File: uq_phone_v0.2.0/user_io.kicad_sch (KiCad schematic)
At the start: 23 parts, among them J8 MCS-302S-C1, M1 C08-00A, Q3 S8050, Q6 MMBT3904LP-7, U10 TPD8F003DQDR, U11 LSM6DSVTR, U12 DRV2603RUNR, U7 TPS22964CYZPR, U8 TPD3F303DQDR

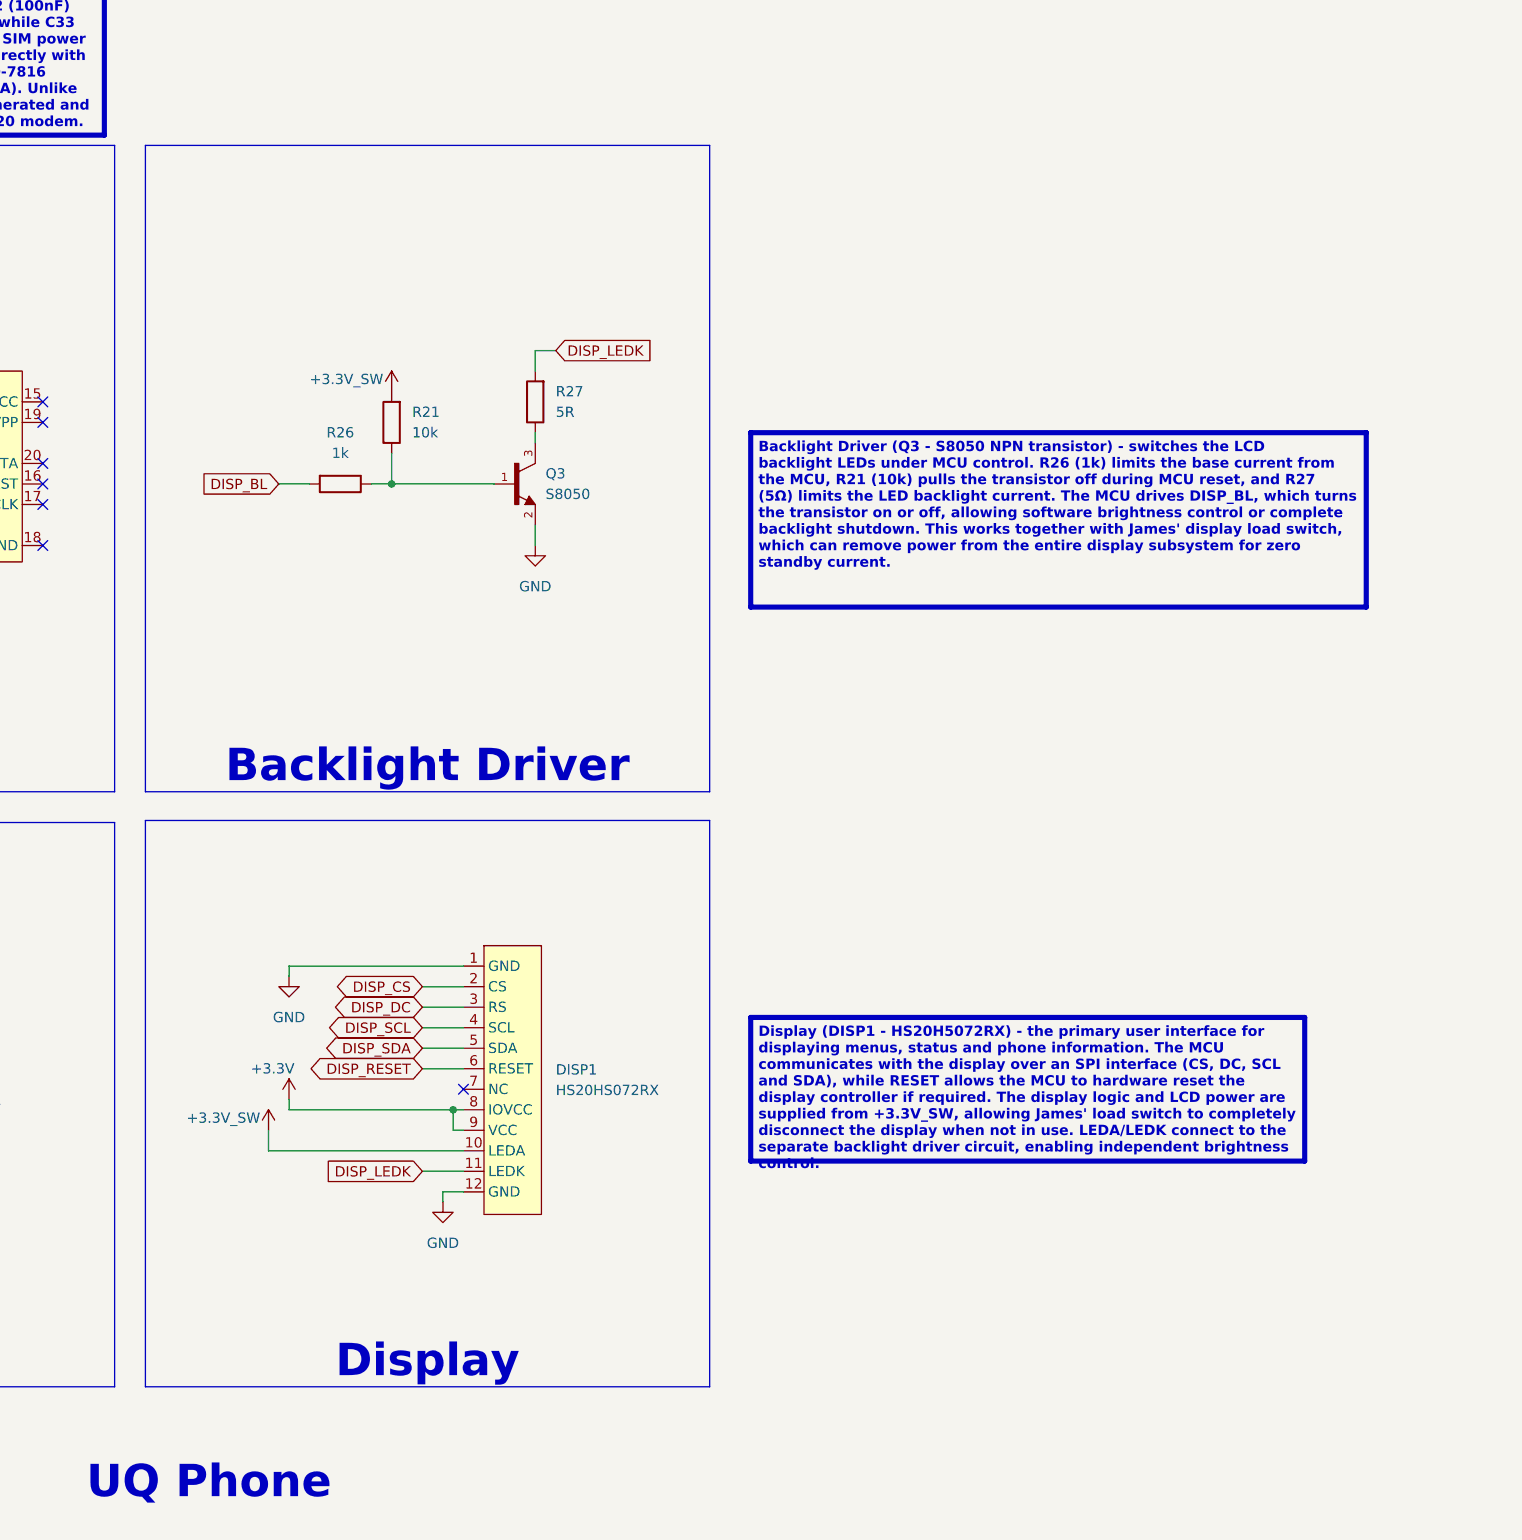
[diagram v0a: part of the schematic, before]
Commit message: new display work
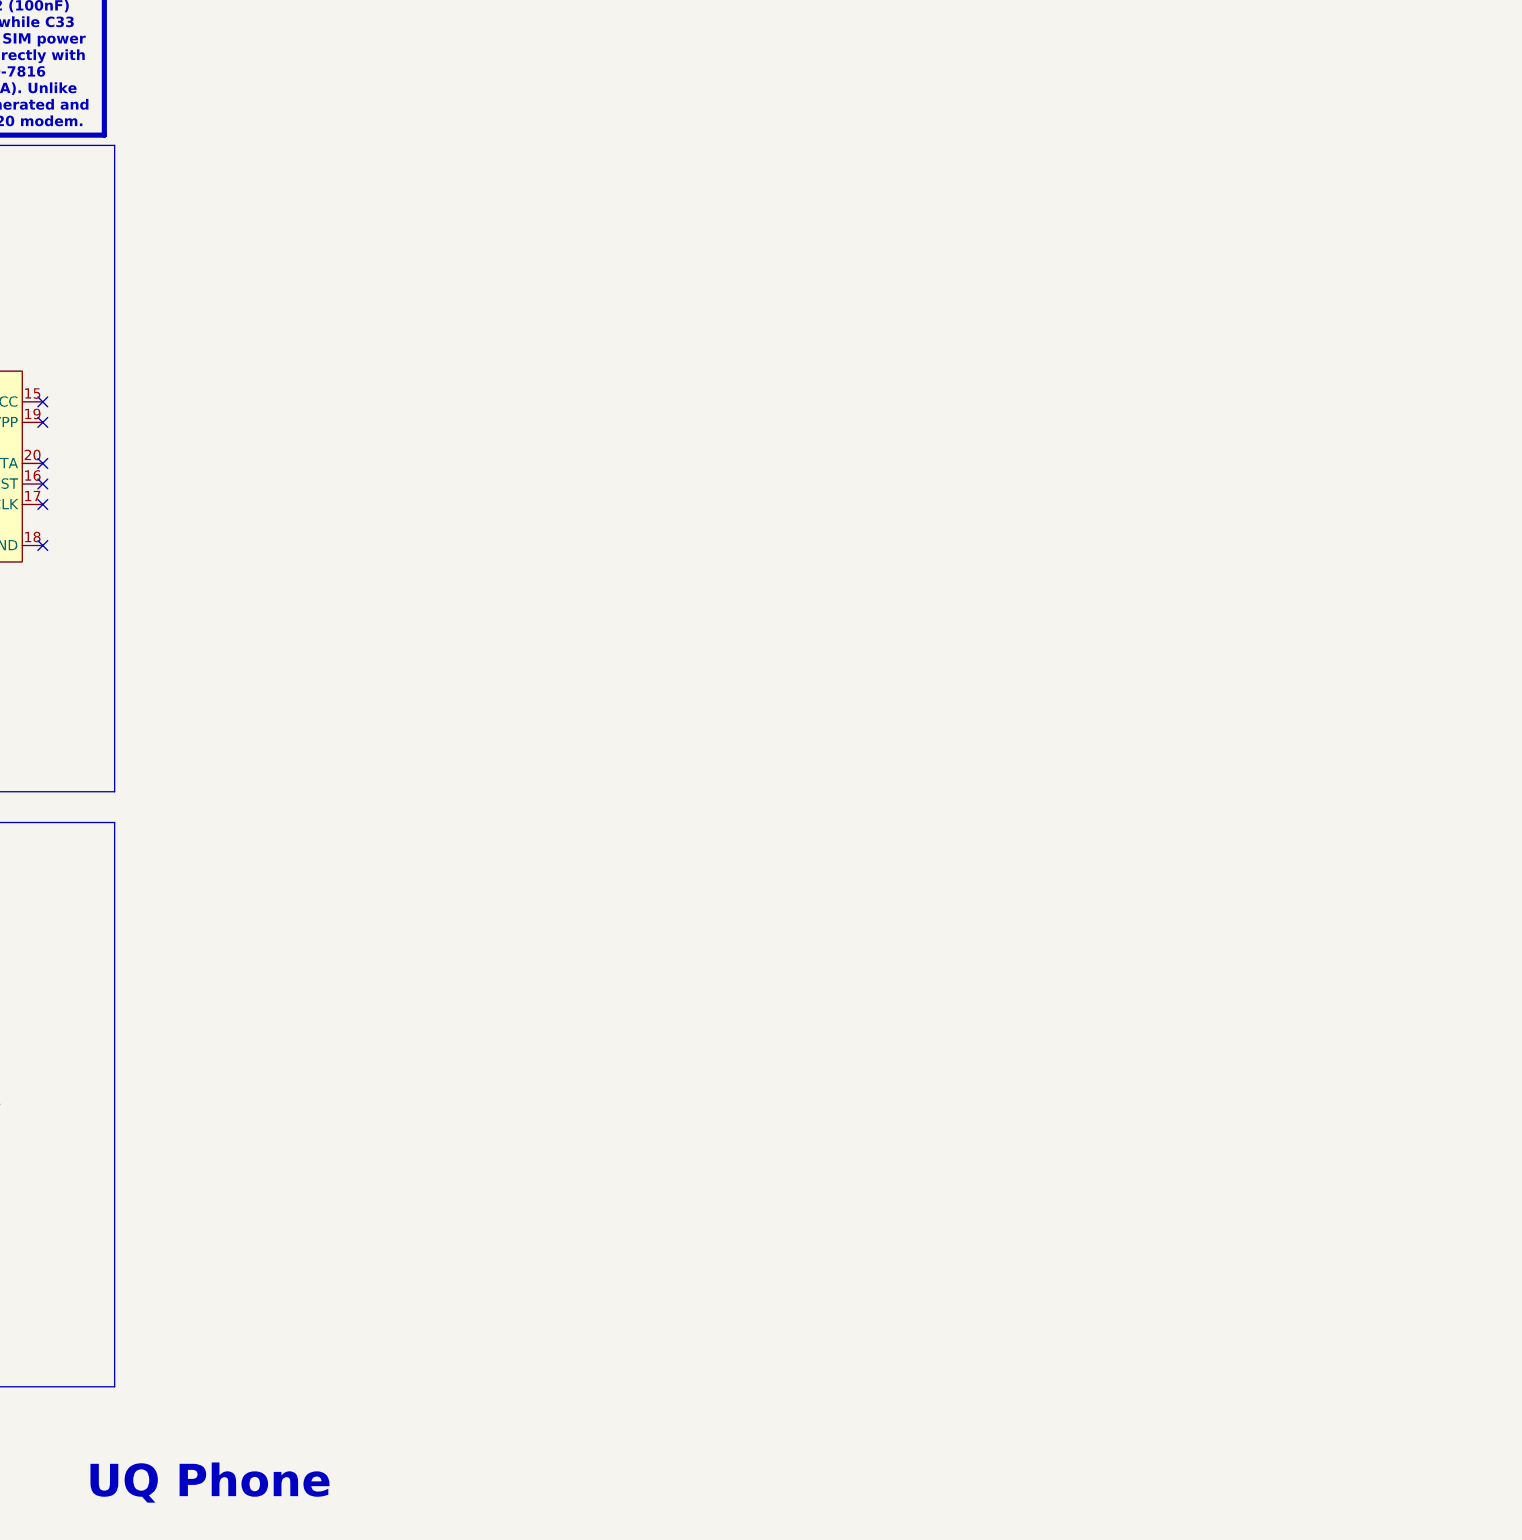
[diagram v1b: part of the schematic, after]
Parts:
- removed DISP1: HS20HS072RX, custom_footprints:Display, symbol Misc:HS20HS072RX
- removed Q3: S8050, Package_TO_SOT_SMD:SOT-23, symbol Misc:S8050
- removed R21: 10k, Resistor_SMD:R_0201_0603Metric, symbol Resistors:Resistor_10k
- removed R26: 1k, Resistor_SMD:R_0402_1005Metric, symbol Resistors:Resistor_1k
- removed R27: 5R, Resistor_SMD:R_0402_1005Metric, symbol Resistors:Resistor_5R
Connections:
- no-connect marks 14 -> 13
